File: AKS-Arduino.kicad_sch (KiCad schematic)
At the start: 9 parts, among them J1 Jack-DC, J2 Conn_01x07_Socket, U1 ATmega328-P, Y1 Crystal

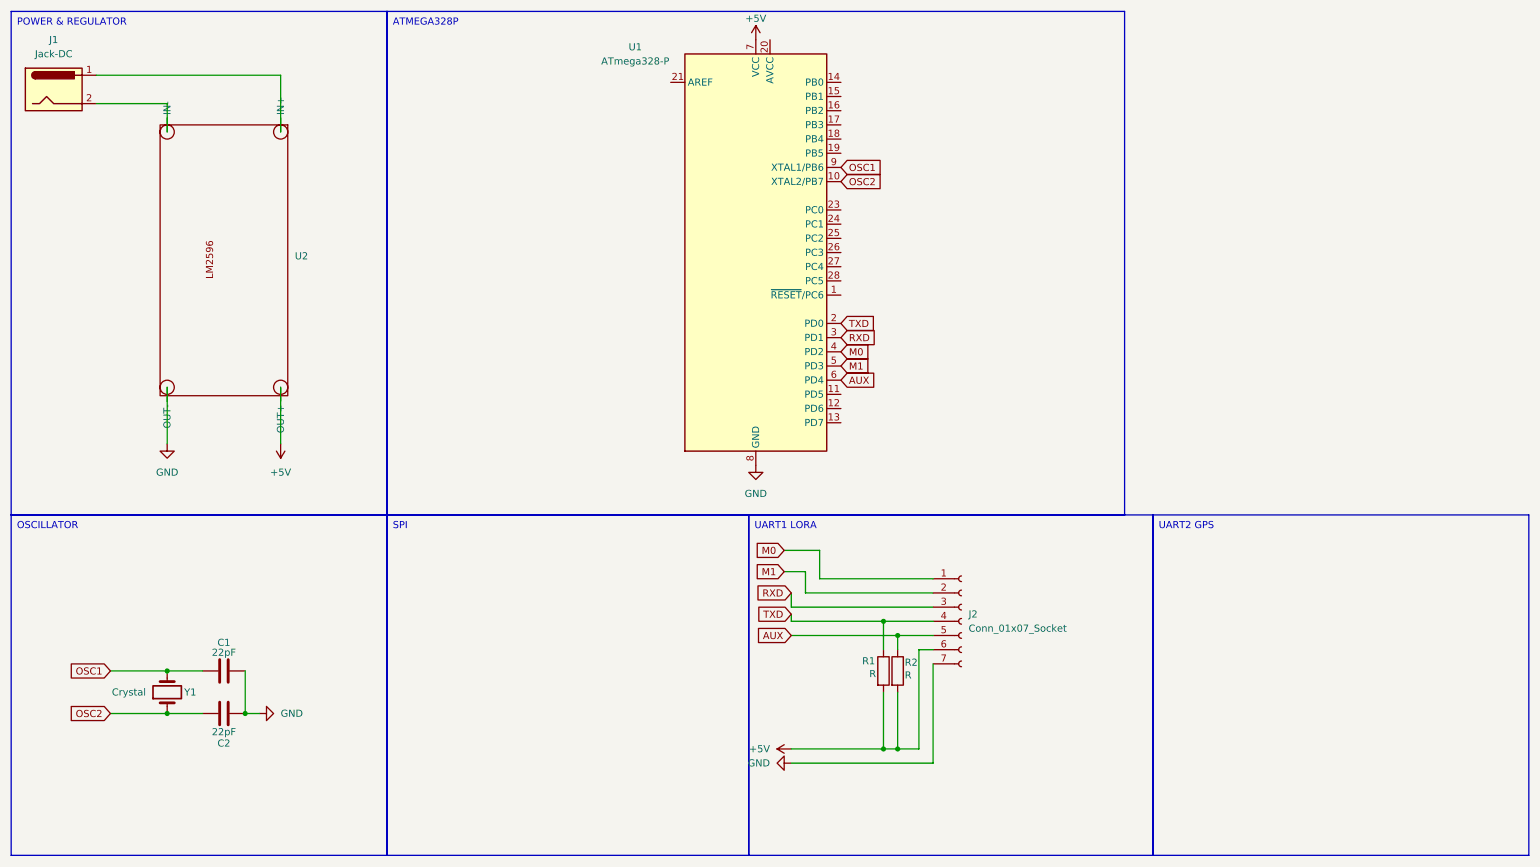
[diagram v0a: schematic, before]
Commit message: Modules added
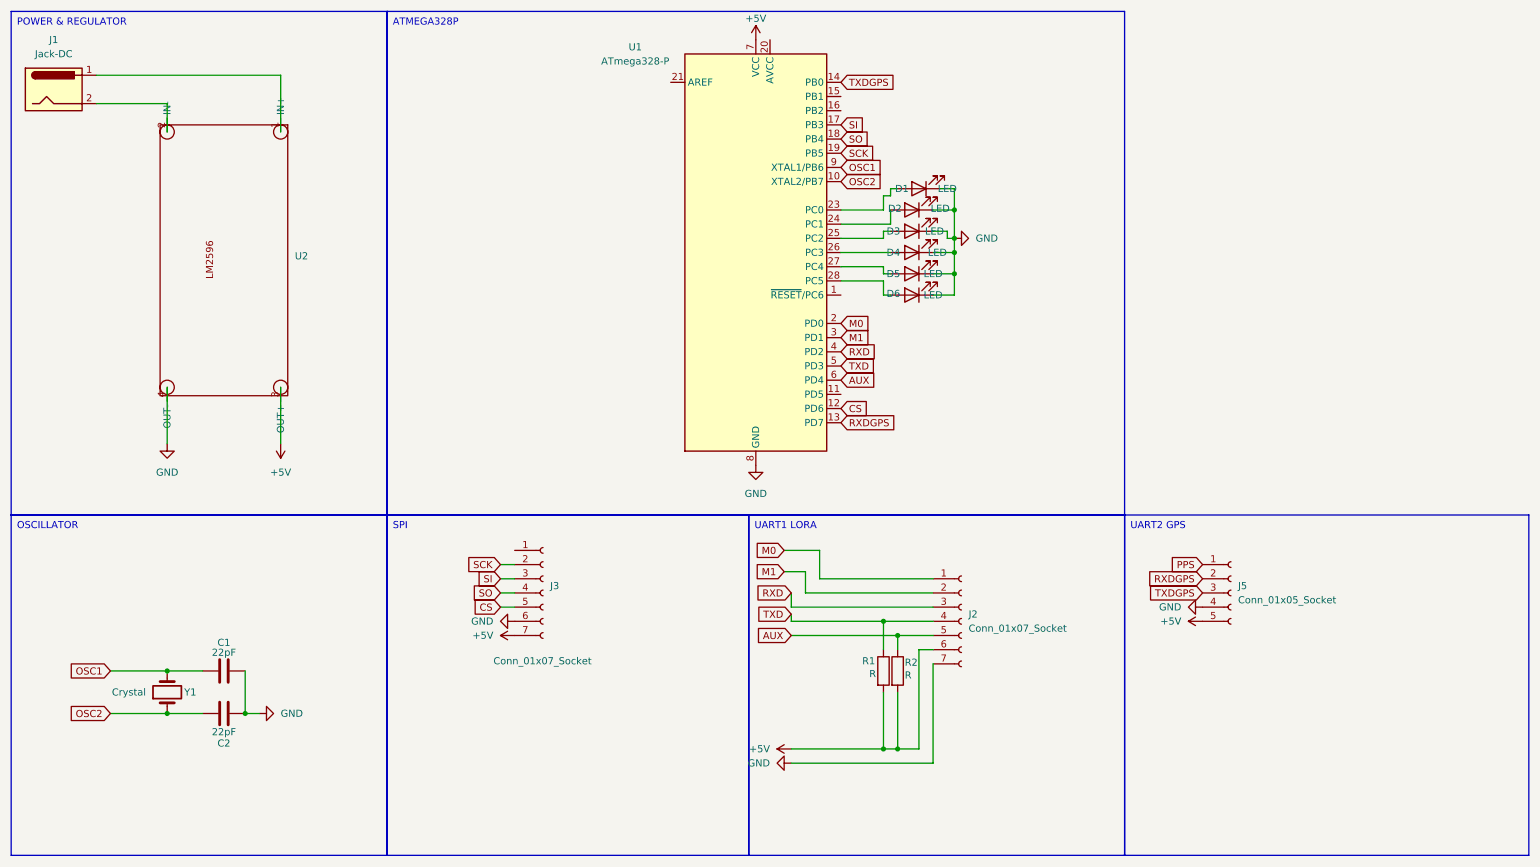
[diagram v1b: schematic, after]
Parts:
- added D1, D2, D3, D4, D5, D6: LED, LED_THT:LED_D3.0mm, symbol Device:LED
- added J3: Conn_01x07_Socket, Connector_PinHeader_2.54mm:PinHeader_1x07_P2.54mm_Vertical, symbol Connector:Conn_01x07_Socket
- added J5: Conn_01x05_Socket, Connector_PinHeader_2.54mm:PinHeader_1x05_P2.54mm_Vertical, symbol Connector:Conn_01x05_Socket
- C1, C2: footprint (none) -> Capacitor_THT:CP_Radial_D4.0mm_P1.50mm
- J1: footprint (none) -> Connector_BarrelJack:BarrelJack_Horizontal
- J2: footprint (none) -> Connector_PinHeader_2.54mm:PinHeader_1x07_P2.54mm_Vertical
- R1, R2: footprint (none) -> Resistor_THT:R_Axial_DIN0207_L6.3mm_D2.5mm_P5.08mm_Vertical
- U2: footprint (none) -> cls:regulator
- Y1: footprint (none) -> Crystal:Crystal_HC49-4H_Vertical
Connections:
- net +5V: now also U2.3 (OUT+), J3.7 (Pin_7), J5.5 (Pin_5); no longer U2. (OUT-)
- net GND: now also U2.4 (OUT-), D1.1 (K), D2.1 (K), D3.1 (K), D4.1 (K), D5.1 (K), D6.1 (K), J3.6 (Pin_6), J5.4 (Pin_4); no longer U2. (OUT-)
- net M0: now also U1.2 (PD0); no longer U1.4 (PD2)
- net M1: now also U1.3 (PD1); no longer U1.5 (PD3)
- net RXD: now also U1.4 (PD2); no longer U1.3 (PD1)
- net TXD: now also U1.5 (PD3); no longer U1.2 (PD0)
- net at J1.1: now also U2.1 (IN+); no longer U2. (OUT-)
- net at J1.2: now also U2.2 (IN-); no longer U2. (OUT-)
- net CS: now reaches U1.12 (PD6)
- net CS: now also J3.5 (Pin_5)
- net RXDGPS: now reaches U1.13 (PD7)
- net RXDGPS: now also J5.2 (Pin_2)
- net TXDGPS: now reaches U1.14 (PB0)
- net TXDGPS: now also J5.3 (Pin_3)
- net SI: now reaches U1.17 (PB3)
- net SI: now also J3.3 (Pin_3)
- net SO: now reaches U1.18 (PB4)
- net SO: now also J3.4 (Pin_4)
- net SCK: now reaches U1.19 (PB5)
- net SCK: now also J3.2 (Pin_2)
- net at U1.23 (PC0): now also D1.2 (A)
- net at U1.24 (PC1): now also D2.2 (A)
- net at U1.25 (PC2): now also D3.2 (A)
- net at U1.26 (PC3): now also D4.2 (A)
- net at U1.27 (PC4): now also D5.2 (A)
- net at U1.28 (PC5): now also D6.2 (A)
- new net PPS: J5.1 (Pin_1)
